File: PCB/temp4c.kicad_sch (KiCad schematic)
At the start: 43 parts, among them J1 10-24VAC, J2 USB_IN, J3 eflashy32, J4 THERMO1, J5 THERMO2, J6 THERMO3, J7 THERMO4, U1 VXO7803-500, U2 ESP32-WROOM-32D, U3 SHT35-DISB, U4 MAX31855KASA, U5 MAX31855KASA, U6 MAX31855KASA, U7 MAX31855KASA

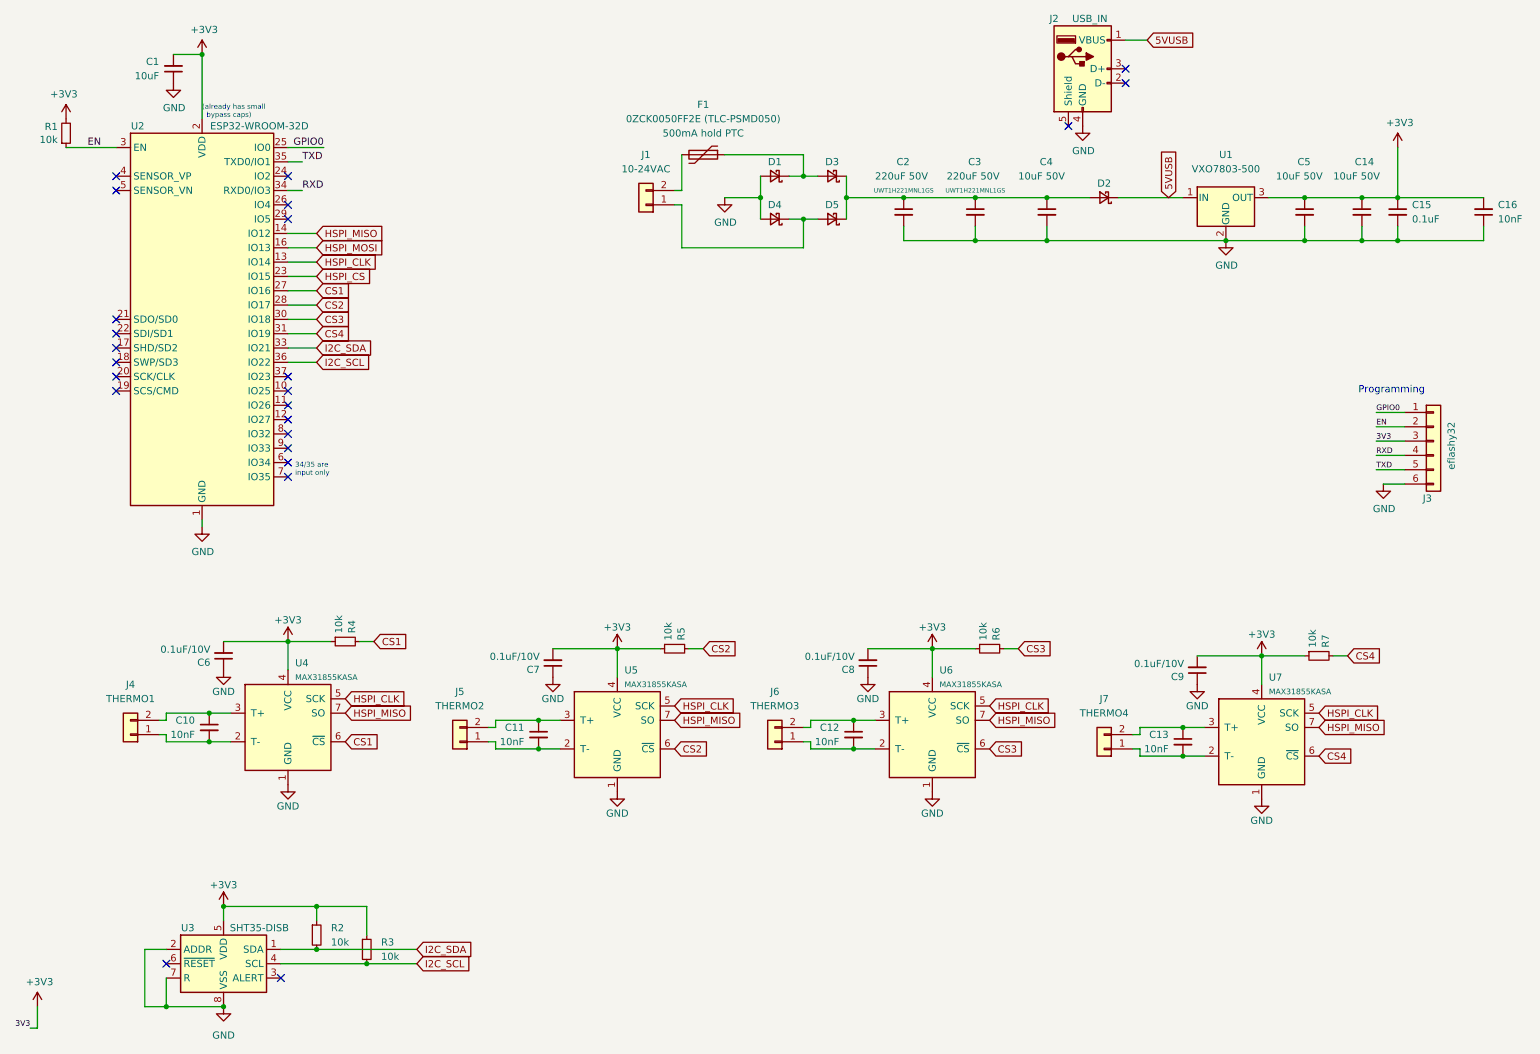
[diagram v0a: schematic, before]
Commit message: Tidy/labels
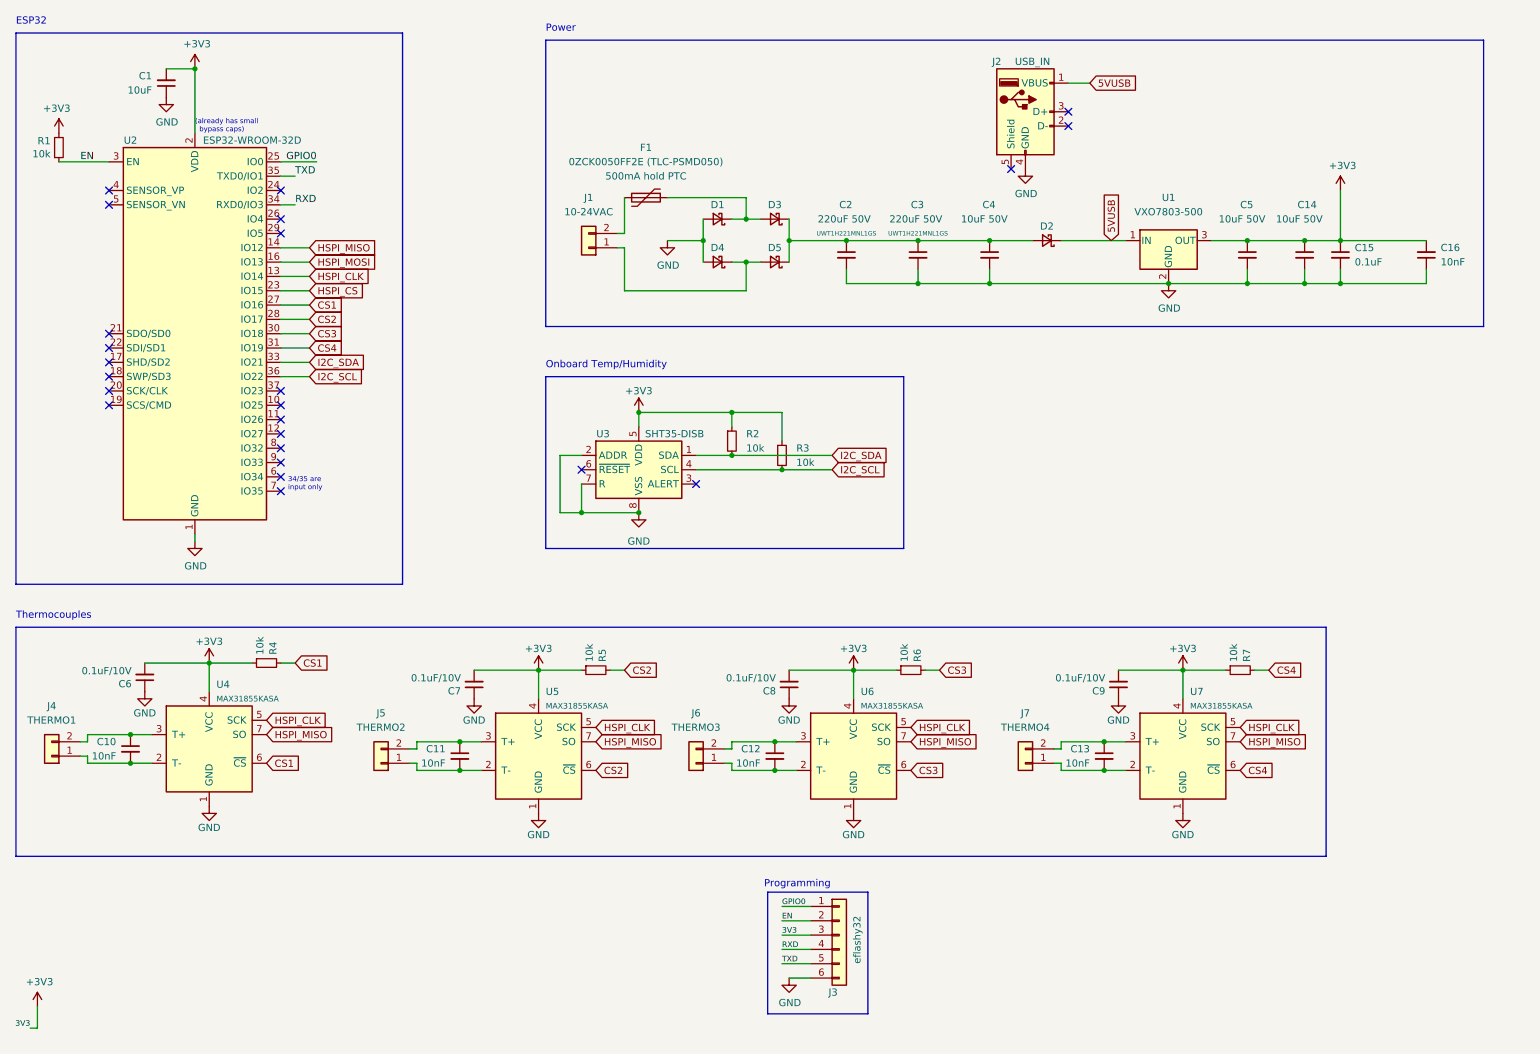
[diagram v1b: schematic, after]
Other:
- note added: "ESP32"
- note added: "Onboard Temp/Humidity"
- note added: "Power"
- note added: "Thermocouples"
- moved on the sheet: C1, C10, C11, C12, C13, C14, C15, C16, C2, C3, C4, C5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
